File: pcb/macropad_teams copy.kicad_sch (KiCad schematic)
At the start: 32 parts, among them J1 Conn_01x04, SW1 SW_Push, SW10 SW_Push, SW11 SW_Push, SW12 SW_Push, SW13 SW_Push, SW14 SW_Push, SW2 SW_Push, SW3 SW_Push, SW4 SW_Push, SW5 SW_Push, SW6 SW_Push, SW7 SW_Push, SW8 SW_Push, SW9 SW_Push, U1 RP2040-ZERO

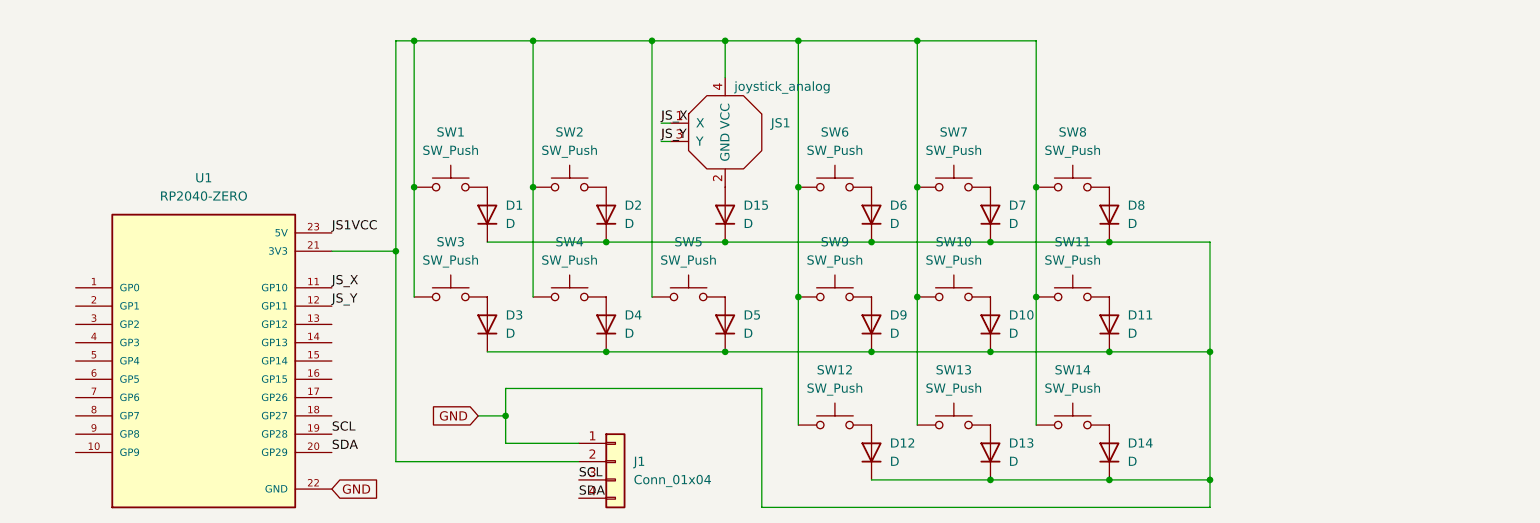
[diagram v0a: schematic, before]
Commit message: modified:   .DS_Store 	new file:   firmware/.DS_Store 	modified:   pcb/.DS_Store 	modified:   pcb/fp-info-cache 	new file:   pcb/macropad_teams copy.kicad_sch deleted:    pcb/macropad_teams-backups/macropad_teams-2025-11-01_171740.zip 	deleted:    pcb/macropad_teams-backups/macropad_teams-2025-11-01_173952.zip 	deleted:    pcb/macropad_teams-backups/macropad_teams-2025-11-01_174521.zip 	deleted:    pcb/macropad_teams-backups/macropad_teams-2025-11-01_175104.zip 	modified:   pcb/macropad_teams.kicad_pcb 	modified:   pcb/macropad_teams.kicad_sch 	new file:   pcb/macropad_teams_manygndvcc.kicad_pcb
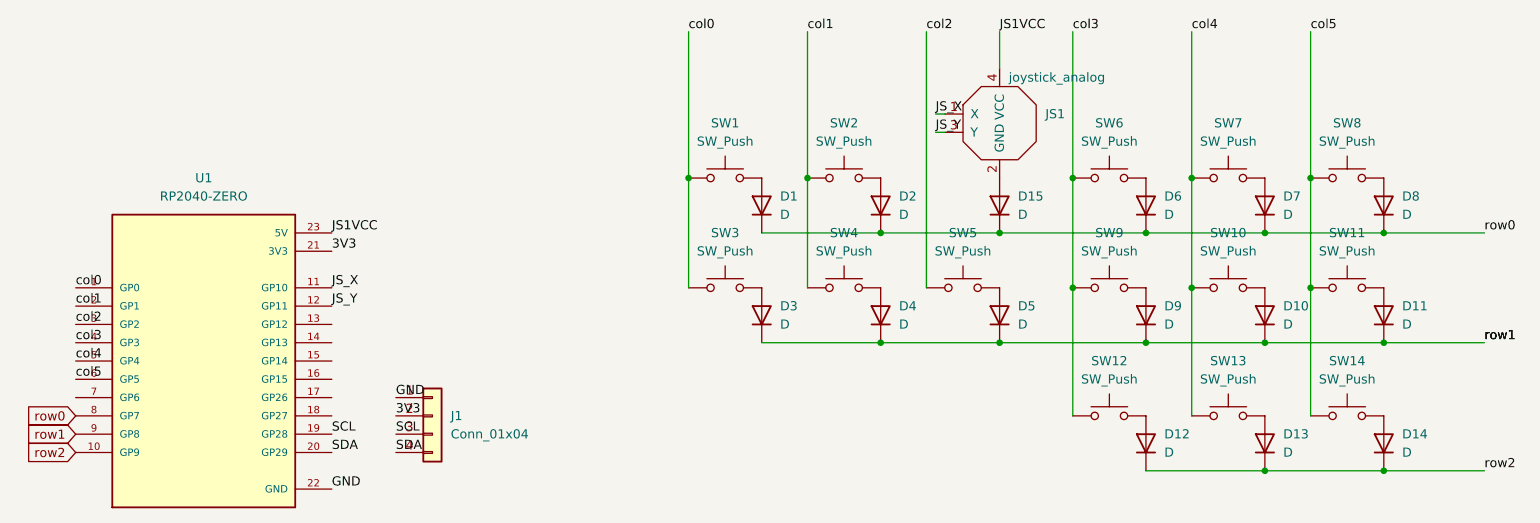
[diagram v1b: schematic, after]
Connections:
- net GND: no longer D1.1 (K), D10.1 (K), D11.1 (K), D12.1 (K), D13.1 (K), D14.1 (K), D15.1 (K), D2.1 (K), D3.1 (K), D4.1 (K), D5.1 (K), D6.1 (K), D7.1 (K), D8.1 (K), D9.1 (K)
- net JS1VCC: now also JS1.4 (VCC)
- net col0: now reaches U1.1 (GP0)
- net col0: now also SW1.1, SW3.1
- net row2: now reaches U1.10 (GP9)
- net row2: now also D12.1 (K), D13.1 (K), D14.1 (K)
- net col1: now reaches U1.2 (GP1)
- net col1: now also SW2.1, SW4.1
- net col2: now reaches U1.3 (GP2)
- net col2: now also SW5.1
- net col3: now reaches U1.4 (GP3)
- net col3: now also SW12.1, SW6.1, SW9.1
- net col4: now reaches U1.5 (GP4)
- net col4: now also SW10.1, SW13.1, SW7.1
- net col5: now reaches U1.6 (GP5)
- net col5: now also SW11.1, SW14.1, SW8.1
- net row0: now reaches U1.8 (GP7)
- net row0: now also D1.1 (K), D15.1 (K), D2.1 (K), D6.1 (K), D7.1 (K), D8.1 (K)
- net row1: now reaches U1.9 (GP8)
- net row1: now also D10.1 (K), D11.1 (K), D3.1 (K), D4.1 (K), D5.1 (K), D9.1 (K)
- new net 3V3: J1.2 (Pin_2), U1.21 (3V3)
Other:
- moved on the sheet: D1, D10, D11, D12, D13, D14, D15, D2, D3, D4, D5, D6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
